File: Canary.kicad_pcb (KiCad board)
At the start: 4 copper layers, 56 x 38 mm, 82 parts, among them J1 CONN_ARM_CM_JTAG_SWD_10, J2 BMD-300-A-R, J3 CONN_20021311-00010T4LF_AMP, J4 USB4125-GF-A, J5 S2B-PH-SM4-TB, Q1 PMN30UNX, Q2 PMN42XPEAH, Q3 PMN30UNX, SW1 TL3301SPF160QJ, U1 DNP, U10 MCP73831T-2ATI_OT, U11 MIC2288YD5, U2 SHTC3, U3 SGP40, U4 MAX6071BAUT21T, U5 LMP91000, U6 SPEC-110-902, U7 MCP6041T-I_OT, U8 RT6150AGQW, U9 LP5907MFX-3.2, Y1 32.7680 kHz

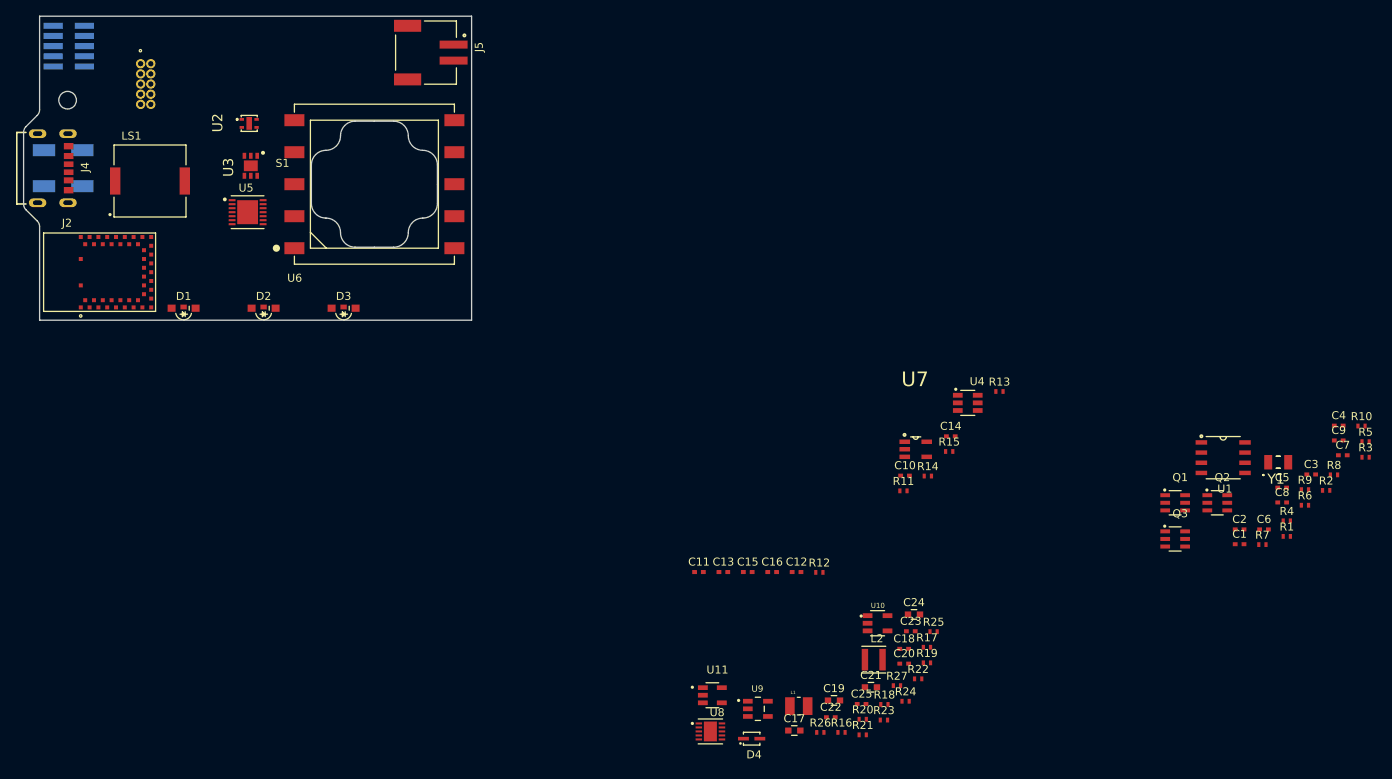
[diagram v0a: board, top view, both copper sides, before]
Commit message: Board setup and rules
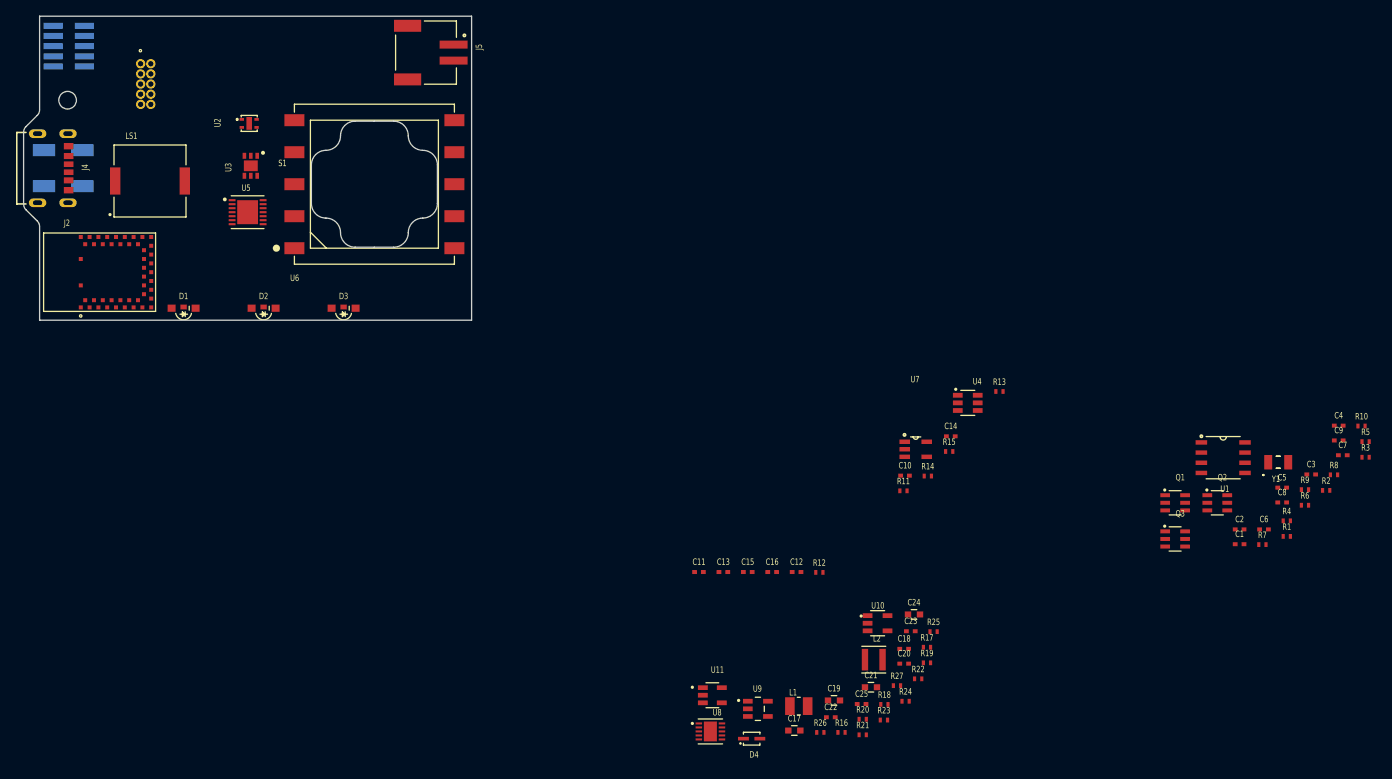
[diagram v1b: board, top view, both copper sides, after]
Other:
- net class Default: clearance 0.2 -> 0.1524; trace_width 0.25 -> 0.1524
- rule trace_clearance: 0.2 -> 0.1524
- rule trace_min: 0.2 -> 0.1524
- rule via_min_size: 0.4 -> 0.6
